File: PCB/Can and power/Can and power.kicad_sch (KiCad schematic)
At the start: 32 parts, among them IC1 MCP2515-e_ST, IC2 TJA1044VT_3Z, J1 TPS54232DR, J2 ESP32, J3 12V, J4 C_H, J5 C_L, J6 GND, Y1 16MHz

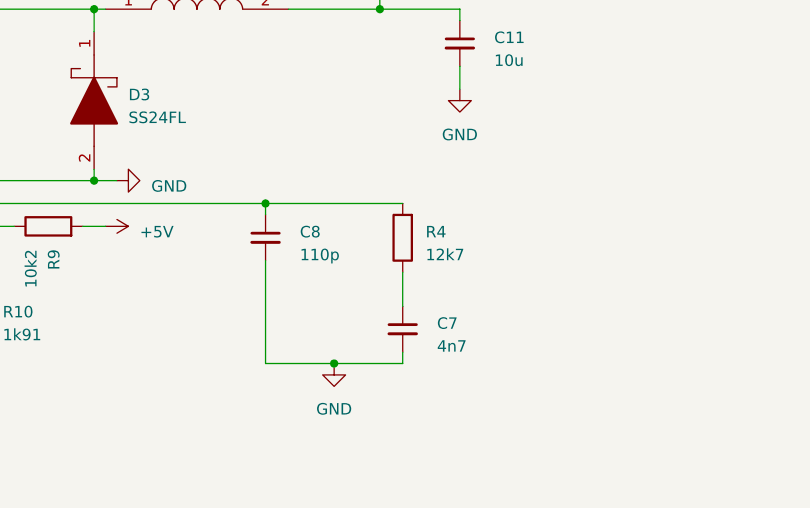
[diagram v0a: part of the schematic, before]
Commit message: Pre-traces
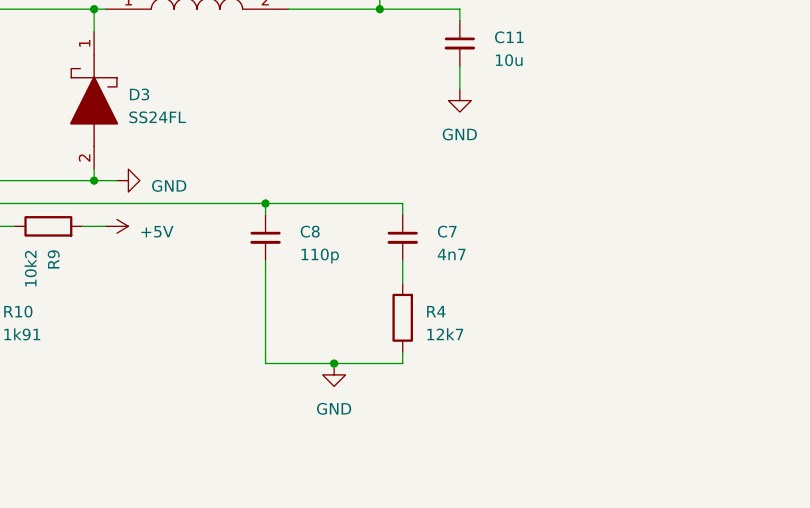
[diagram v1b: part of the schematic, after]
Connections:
- net GND: now also R4.1; no longer C7.2
- net at C7.1: now also C8.1, J1.6 (COMP); no longer R4.1
- new net: C7.2, R4.2
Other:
- moved on the sheet: C7, R4
